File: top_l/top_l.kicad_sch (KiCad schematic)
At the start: 57 parts, among them J1 Conn_01x02_Pin, SW1 SW_Push, SW10 SW_Push, SW11 SW_Push, SW12 SW_Push, SW13 SW_Push, SW14 SW_Push, SW15 SW_Push, SW16 SW_Push, SW17 SW_Push, SW18 SW_Push, SW19 SW_Push, SW2 SW_Push, SW20 SW_Push, SW21 SW_Push, SW22 SW_Push, SW23 SW_Push, SW24 SW_Push, SW25 SW_Push, SW26 SW_Push, SW27 SW_Push, SW28 SW_Push, SW3 SW_Push, SW4 SW_Push, SW5 SW_Push, SW6 SW_Push, SW7 SW_Push, SW8 SW_Push, SW9 SW_Push, U1 Micon_BLEMicroPro

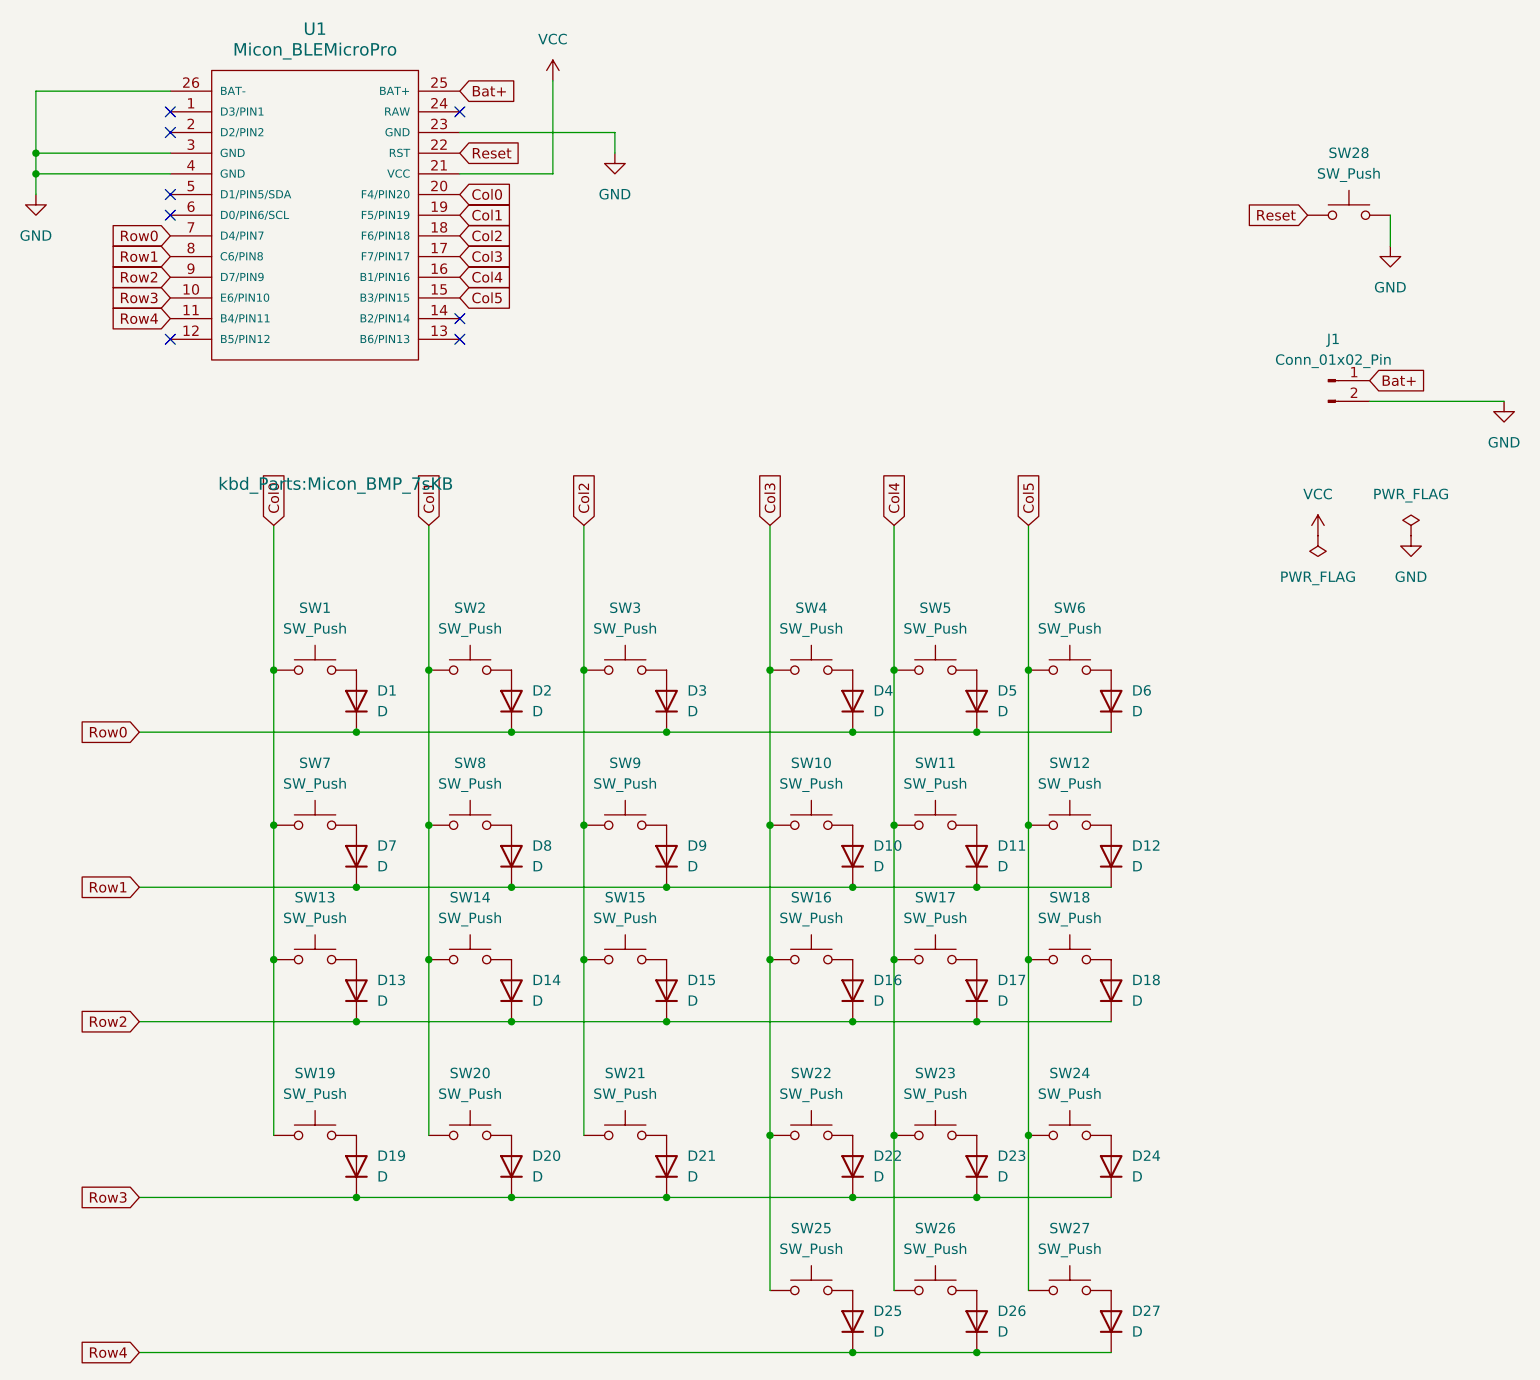
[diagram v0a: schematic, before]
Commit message: refactor: top left plate
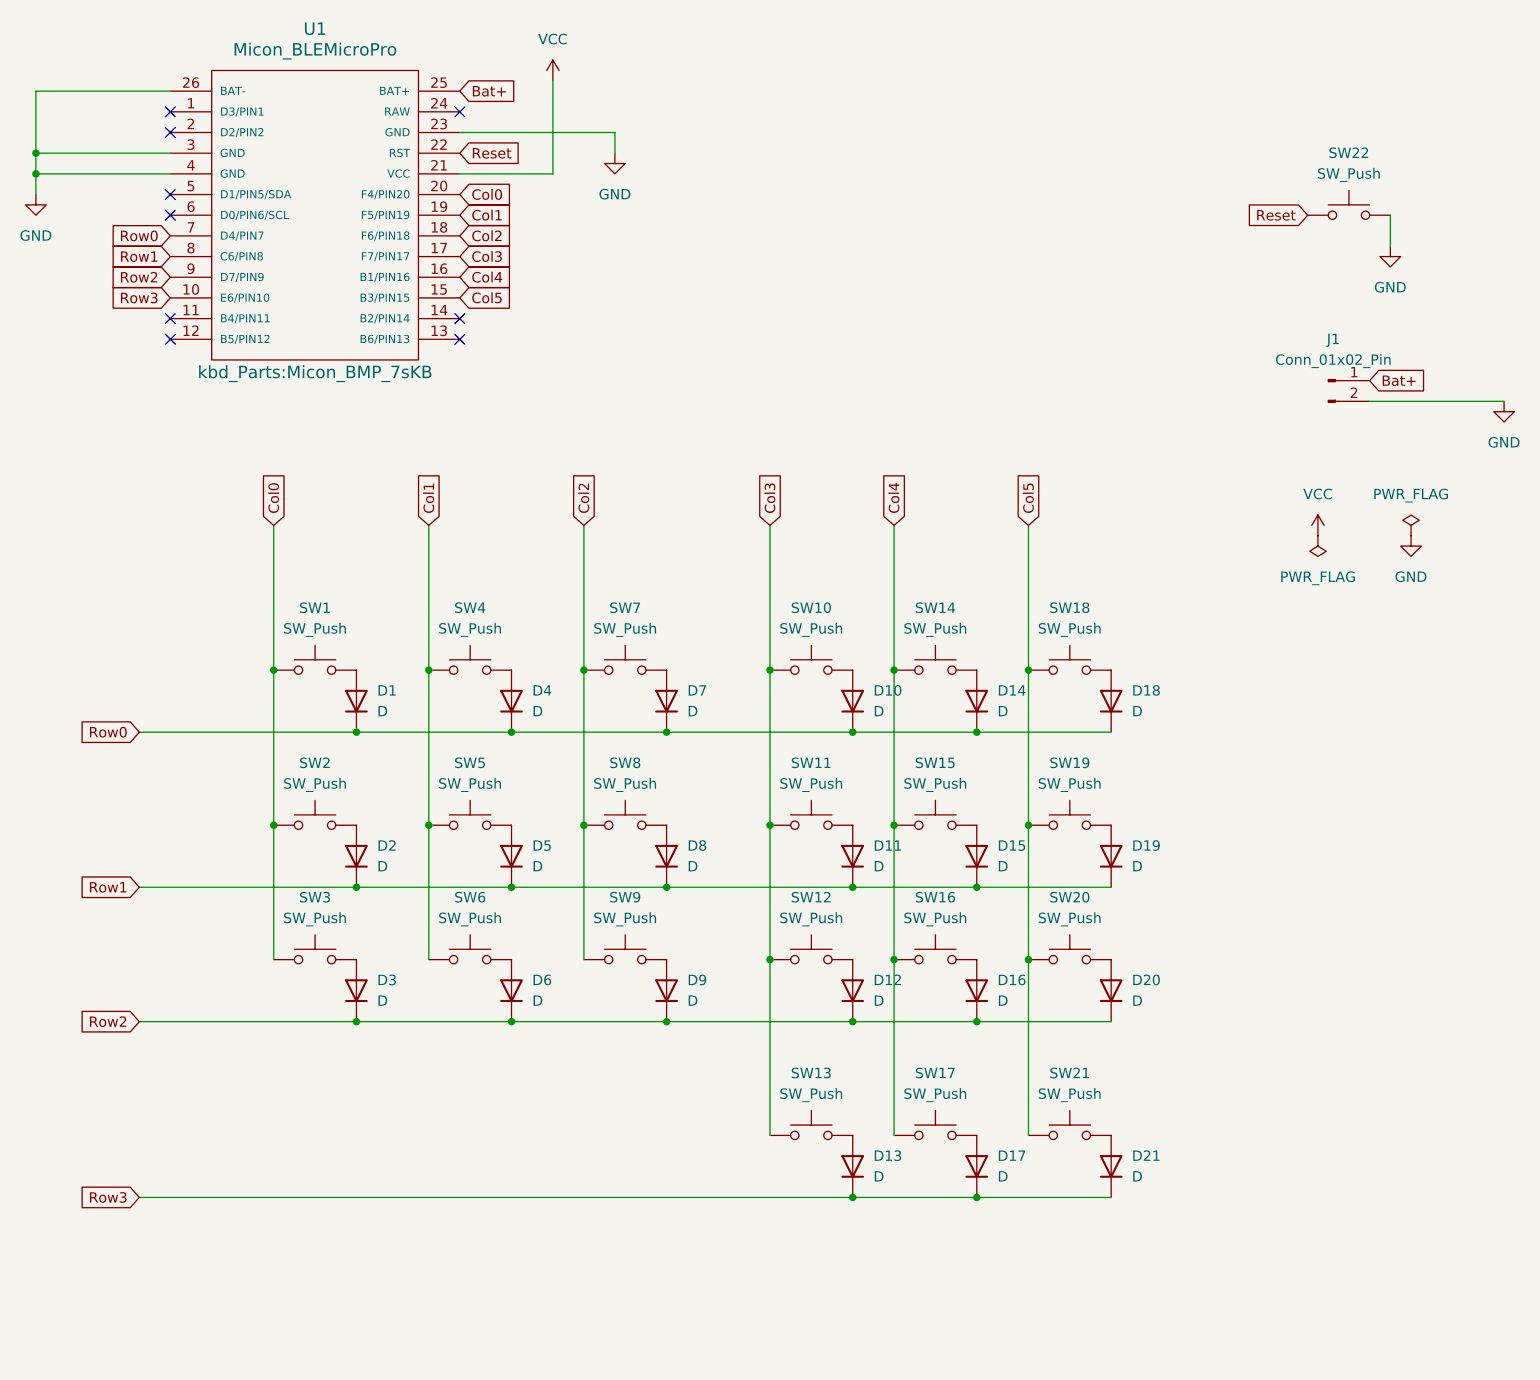
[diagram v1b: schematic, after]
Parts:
- removed D19, D20, D21, D22, D23, D24: D, kbd_Parts:Diode_TH_SMD, symbol Device:D
- removed SW19, SW20, SW21, SW22, SW23, SW24: SW_Push, kbd_SW:Choc_v2_Hotswap_1u_16.5, symbol Switch:SW_Push
- renumbered D4 to D10, D10 to D11, D16 to D12, D25 to D13, D5 to D14, D11 to D15, D17 to D16, D26 to D17, D6 to D18, D12 to D19, D7 to D2, D18 to D20, D27 to D21, D13 to D3, D2 to D4, D8 to D5, D14 to D6, D3 to D7, D9 to D8, D15 to D9, SW4 to SW10, SW10 to SW11, SW16 to SW12, SW25 to SW13, SW5 to SW14, SW11 to SW15, SW17 to SW16, SW26 to SW17, SW6 to SW18, SW12 to SW19, SW7 to SW2, SW18 to SW20, SW27 to SW21, SW28 to SW22, SW13 to SW3, SW2 to SW4, SW8 to SW5, SW14 to SW6, SW3 to SW7, SW9 to SW8, SW15 to SW9
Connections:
- net Row3: now also D13.1 (K), D17.1 (K), D21.1 (K)
- removed net Row4: D13.1 (K), D17.1 (K), D21.1 (K), U1.11 (B4/PIN11)
- no-connect marks 8 -> 9
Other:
- moved on the sheet: D13, D17, D21, SW13, SW17, SW21
